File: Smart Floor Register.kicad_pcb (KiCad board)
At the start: 2 copper layers, 115.9 x 79.2 mm, 68 parts, among them J1 Fan 1, J2 Fan 2, J3 USB_B_Micro, J4 AVR-ISP-6, M1 Motor_Servo, SW1 RESET, SW2 PEN, SW3 Fan, SW4 Servo, U1 ATmega64A-A, U2 AD8539ARMZ-REEL, U3 AD8539ARMZ-REEL, U4 LTC1695, U5 LTC1695, U6 XC9142B50CMR-G, Y1 16MHz

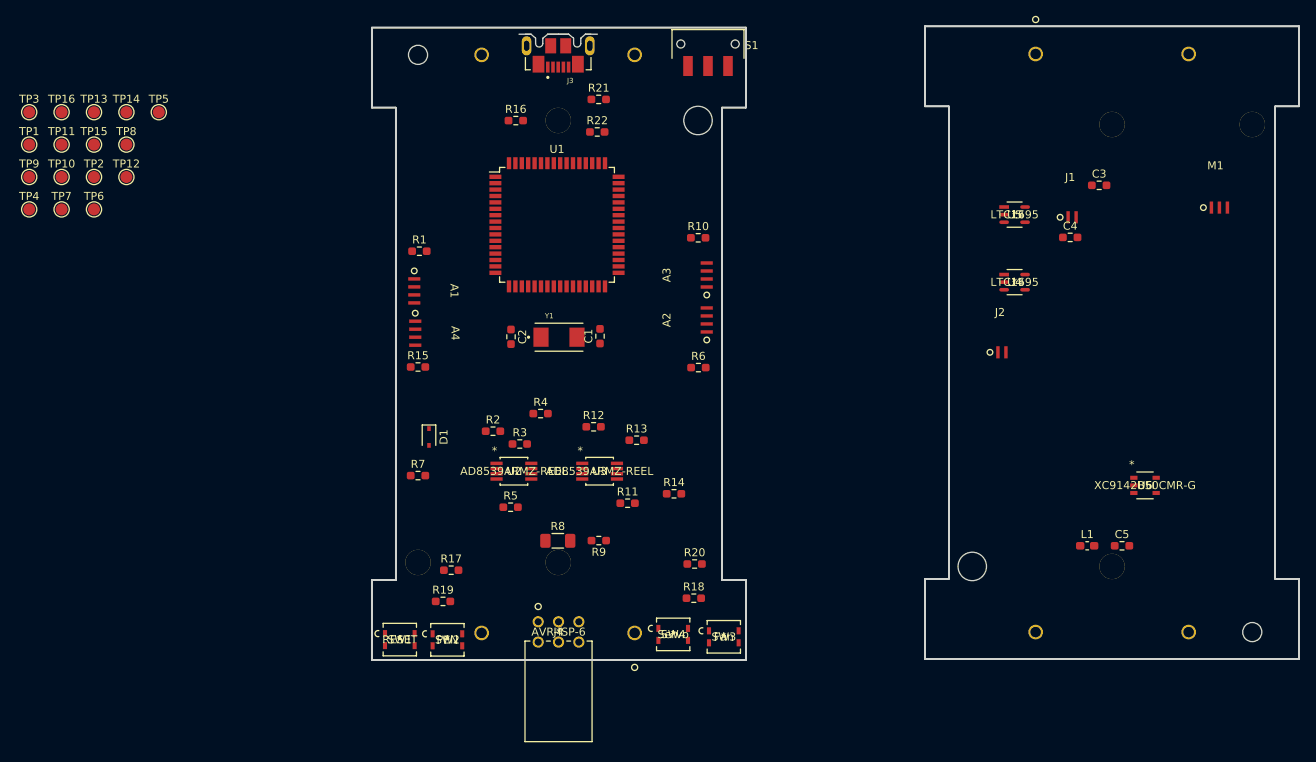
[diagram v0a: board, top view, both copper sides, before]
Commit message: PCB
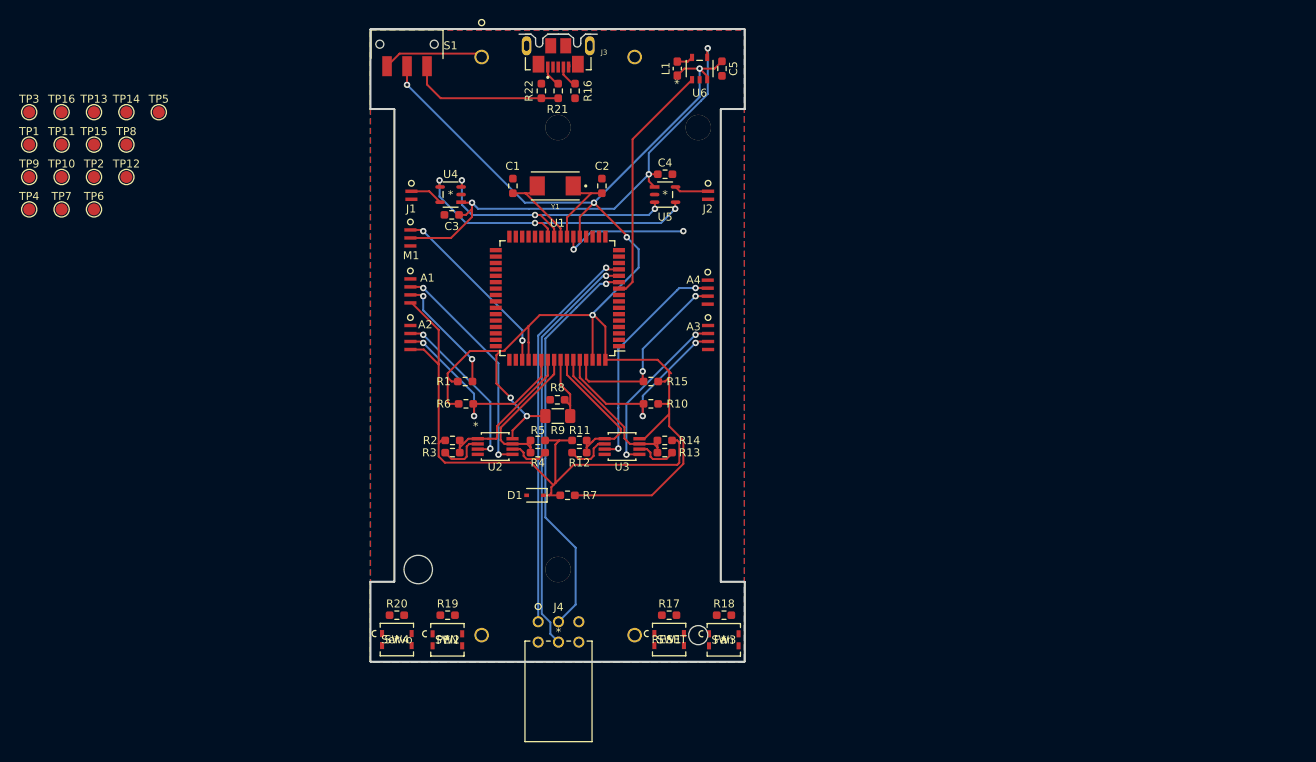
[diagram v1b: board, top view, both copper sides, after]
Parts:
- removed BT1: 18650, SFRFootprints:1049P
- moved M1 96.2 mm to (110.1, 93.6), turned to -90 degrees
- moved C3 81.0 mm to (110.5, 91.2), turned to 180 degrees
- moved L1 78.6 mm to (138.7, 72.9), turned to 90 degrees
- moved J1 77.9 mm to (109.9, 88.5), turned to -90 degrees
- moved C5 77.8 mm to (144.3, 72.9), turned to -90 degrees
- moved U6 76.2 mm to (141.5, 72.9), turned to 90 degrees
- moved BT2 74.5 mm to (114.2, 71.5), turned to -90 degrees
- moved U4 71.3 mm to (110.4, 88.6), turned to 180 degrees
- moved C4 51.3 mm to (137.2, 86.1)
- moved U5 43.8 mm to (137.2, 88.6)
- moved R20 37.8 mm to (103.6, 141.2)
- moved S1 37.6 mm to (104.9, 69.8)
- moved A4 36.9 mm to (147.0, 100.8)
- moved J2 35.5 mm to (147.0, 88.5), turned to -90 degrees
- moved SW4 34.5 mm to (103.6, 144.3)
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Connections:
- U1 pad 54: Thermistor -> ThermistorB
- U1 pad 55: ThermistorA -> ThermopileB
- U1 pad 56: ThermopileC -> ThermopileA
- U1 pad 57: ThermistorD -> Thermistor
- U1 pad 59: ThermistorC -> ThermopileC
- U1 pad 60: ThermopileB -> ThermistorC
- U1 pad 61: ThermopileA -> ThermistorD
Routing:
- net VCC: track 0.00 -> 190.4 mm, vias 0 -> 7
- net Shifted Ground: track 0.00 -> 74.8 mm
- net +5V: track 0.00 -> 61.1 mm, vias 0 -> 3
- net MOSI: track 0.00 -> 51.8 mm, vias 0 -> 1
- net SCK: track 0.00 -> 50.0 mm, vias 0 -> 1
- net MISO: track 0.00 -> 49.5 mm, vias 0 -> 1
- net SDA: track 0.00 -> 38.2 mm, vias 0 -> 3
- net SCL: track 0.00 -> 33.8 mm, vias 0 -> 3
- net MotorEnable: track 0.00 -> 30.4 mm
- net Net-(A4-Pad2): track 0.00 -> 28.5 mm, vias 0 -> 2
- net Net-(A1-Pad2): track 0.00 -> 28.2 mm, vias 0 -> 2
- net ThermistorB: track 0.00 -> 27.9 mm, vias 0 -> 2
- net ThermistorC: track 0.00 -> 26.6 mm, vias 0 -> 2
- net ThermistorD: track 0.00 -> 24.7 mm, vias 0 -> 2
- net ServoPWM: track 0.00 -> 23.0 mm, vias 0 -> 2
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- added copper zone on B.Cu, net Earth
- added copper zone on F.Cu, net Earth
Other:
- board size 115.9 x 79.2 mm -> 46.8 x 79.1 mm

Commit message: PCB
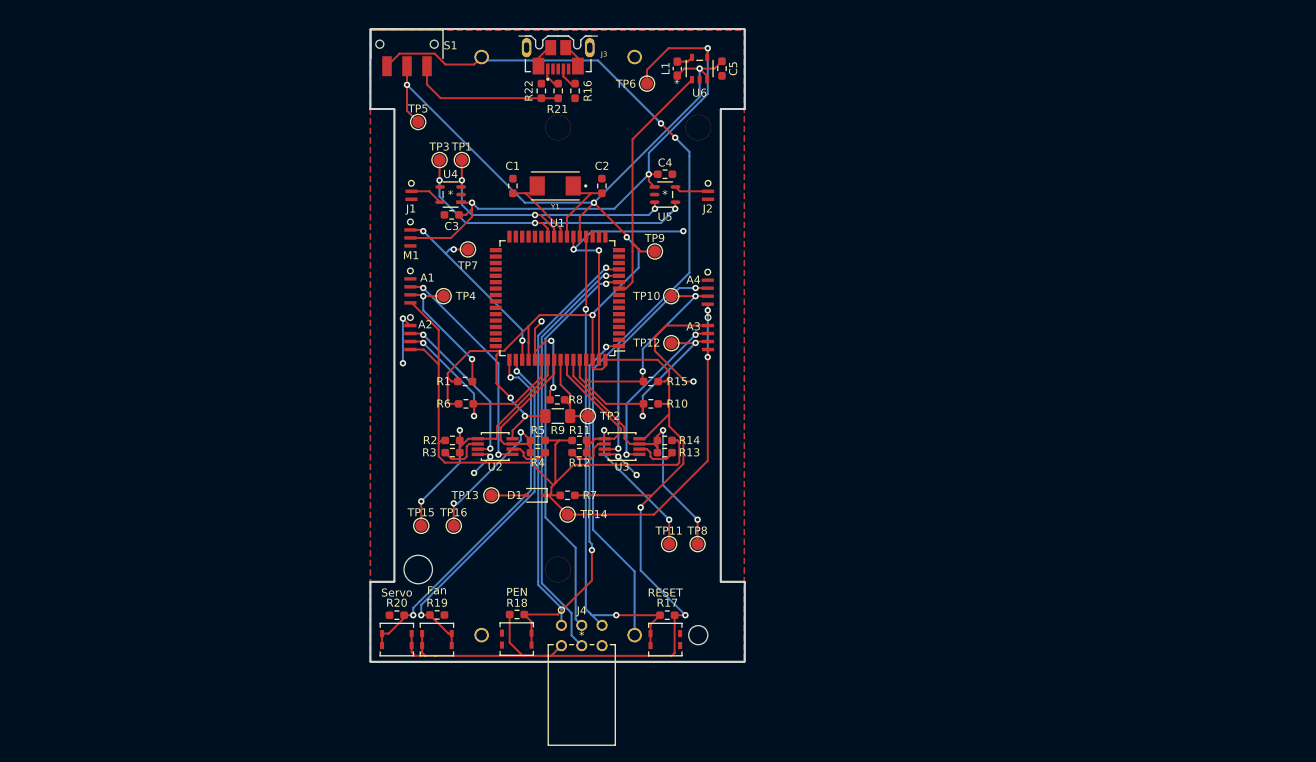
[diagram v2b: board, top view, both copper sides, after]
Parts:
- moved TP11 90.9 mm to (137.7, 132.3)
- moved TP8 87.1 mm to (141.2, 132.3)
- moved TP9 78.8 mm to (135.9, 95.8)
- moved TP10 77.6 mm to (137.9, 101.3)
- moved TP14 74.6 mm to (125.0, 128.7)
- moved TP16 71.2 mm to (110.7, 130.0)
- moved TP12 71.2 mm to (137.9, 107.2)
- moved TP6 70.9 mm to (134.9, 74.8)
- moved TP13 69.0 mm to (115.5, 126.2)
- moved TP2 68.6 mm to (127.5, 116.3)
- moved TP15 62.8 mm to (106.7, 130.0)
- moved TP1 54.1 mm to (111.8, 84.3)
- moved TP4 52.9 mm to (109.5, 101.3)
- moved TP3 51.6 mm to (109.0, 84.3)
- moved TP7 51.0 mm to (112.5, 95.5)
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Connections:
- BT2 pad 3: (no net) -> Earth
- BT2 pad 4: (no net) -> Net-(BT1-Pad1)
- U1 pad 49: FanActivate -> ServoActivate
- U1 pad 50: ServoActivate -> FanActivate
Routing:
- net Net-(BT1-Pad1): track 12.7 -> 111.9 mm, vias 0 -> 2
- net VCC: track 190.4 -> 263.2 mm, vias 7 -> 9
- net Earth: track 20.4 -> 92.9 mm, vias 2 -> 13
- net ~{RESET}: track 0.00 -> 62.9 mm, vias 0 -> 2
- net ServoActivate: track 0.00 -> 46.3 mm, vias 0 -> 2
- net ~{PEN}: track 0.00 -> 46.1 mm, vias 0 -> 2
- net FanActivate: track 0.00 -> 45.1 mm, vias 0 -> 2
- net Shifted Ground: track 74.8 -> 119.2 mm, vias 0 -> 2
- net ThermopileD: track 18.4 -> 37.1 mm, vias 0 -> 2
- net ThermopileC: track 18.6 -> 36.2 mm, vias 0 -> 2
- net ThermopileA: track 18.4 -> 35.5 mm, vias 0 -> 2
- net ThermopileB: track 19.3 -> 34.3 mm, vias 0 -> 2
- net +5V: track 61.1 -> 71.5 mm
- net MotorEnable: track 30.4 -> 33.6 mm
- net ThermistorD: track 24.7 -> 27.7 mm
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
